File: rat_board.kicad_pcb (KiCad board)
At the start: 2 copper layers, 43.2 x 51.4 mm, 55 parts, among them M1 LEFT_MOTOR, M2 RIGHT_MOTOR, SW2 SWITCH_INV, U3 STM32F103C8T6

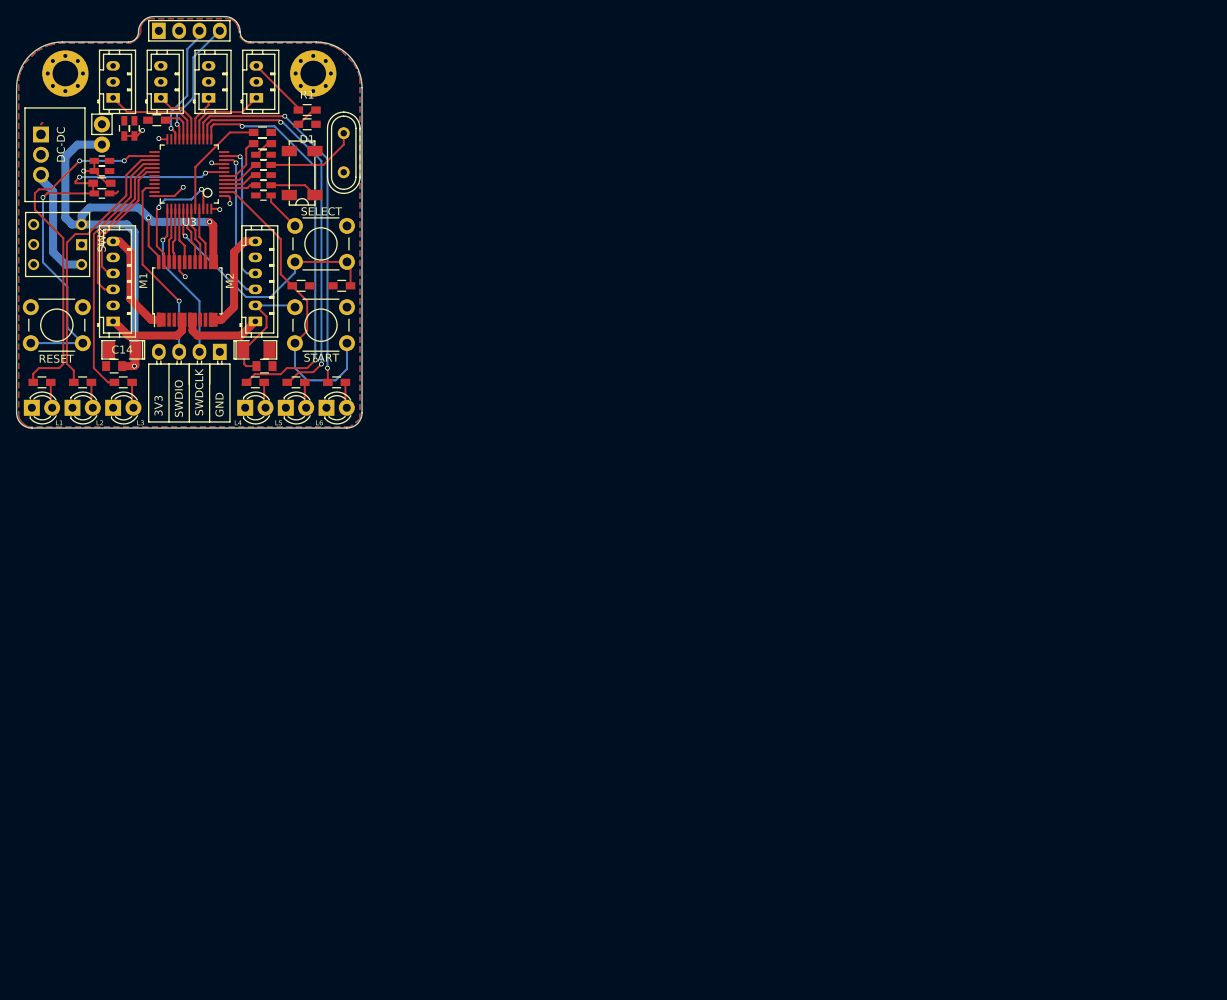
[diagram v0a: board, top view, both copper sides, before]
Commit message: releseable board
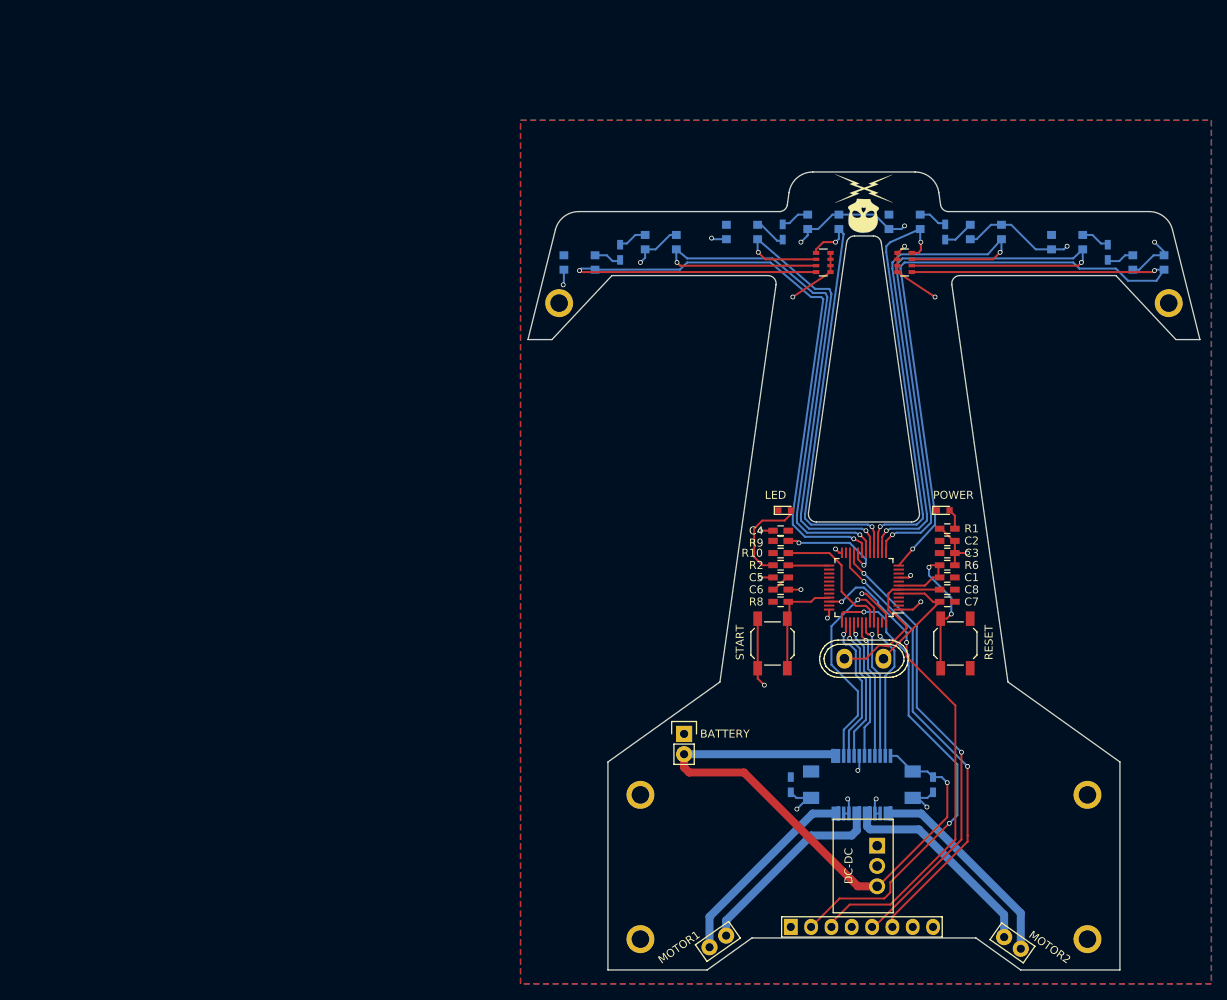
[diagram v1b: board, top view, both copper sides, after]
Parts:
- removed the ? at (75.9, 42.9)
- removed the ? at (45.7, 46.7)
- removed the ? at (38.2, 71.6)
- removed the ? at (43.3, 71.6)
- removed the ? at (48.4, 71.6)
- removed the ? at (64.9, 71.6)
- removed the ? at (75.7, 59.6)
- removed the ? at (70.6, 59.6)
- removed the ? at (65.8, 40.4)
- removed the ? at (70.0, 71.6)
- removed the ? at (75.1, 71.6)
- removed the ? at (52.8, 27.7)
- removed the ? at (65.9, 43.2)
- removed the ? at (65.9, 47.0)
- removed the ? at (65.9, 45.7)
- removed the ? at (65.0, 67.6)
- removed the ? at (45.7, 45.2)
- removed the ? at (45.7, 43.9)
- removed the ? at (65.9, 48.3)
- removed the ? at (49.8, 39.9)
- removed the ? at (48.5, 39.9)
- removed the ? at (65.9, 44.5)
- removed the ? at (45.7, 48.0)
- removed the ? at (65.8, 41.8)
- removed the ? at (52.6, 38.9)
- removed the ? at (47.2, 69.6)
- removed the ? at (66.0, 69.6)
- removed the ? at (60.5, 67.8)
- removed the ? at (41.1, 33.0)
- removed the ? at (56.4, 60.2)
- removed the ? at (70.7, 45.5)
- removed the ? at (38.1, 43.2)
- removed the ? at (72.1, 33.0)
- removed D1: LED_Power, Resistors_SMD:R_0603_HandSoldering
- removed the DC-DC at (45.7, 41.9)
- removed the G*** at (56.1, 45.0)
- removed L1: LED_0, LEDs:LED-3MM
- removed L2: LED_1, LEDs:LED-3MM
- removed L3: LED_2, LEDs:LED-3MM
- removed L4: LED_3, LEDs:LED-3MM
- removed L5: LED_4, LEDs:LED-3MM
- removed L6: LED_5, LEDs:LED-3MM
- removed M1: LEFT_MOTOR, Connectors_JST:JST_PH_B6B-PH-K_06x2.00mm_Straight
- removed M2: RIGHT_MOTOR, Connectors_JST:JST_PH_B6B-PH-K_06x2.00mm_Straight
- removed the RESET at (36.8, 62.2)
- removed S1: FRONT_LEFT_IR, Connectors_JST:JST_PH_B3B-PH-K_03x2.00mm_Straight
- removed S2: SIDE_LEFT_IR, Connectors_JST:JST_PH_B3B-PH-K_03x2.00mm_Straight
- removed S3: SIDE_RIGHT_IR, Connectors_JST:JST_PH_B3B-PH-K_03x2.00mm_Straight
- removed S4: FRONT_RIGHT_IR, Connectors_JST:JST_PH_B3B-PH-K_03x2.00mm_Straight
- removed SELECT: SELECT_BUTTON, Buttons_Switches_ThroughHole:SW_PUSH_6mm
- removed the START at (69.8, 62.2)
- removed SW2: SWITCH_INV, Buttons_Switches_ThroughHole:SW_PUSH_x2
- removed U3: STM32F103C8T6, Housings_QFP:LQFP-48_7x7mm_Pitch0.5mm
- added ?: TB6612FNG, custom-lib:driver_tuneado, B.Cu at (140.7, 121.9)
- added ?: 47k, Resistors_SMD:R_Array_Convex_4x0603, F.Cu at (146.1, 56.6)
- added ?: MountingHole_2.2mm_M2_ISO7380_Pad, Mounting_Holes:MountingHole_2.2mm_M2_ISO7380_Pad, F.Cu at (102.9, 61.7)
- added ?: MountingHole_2.2mm_M2_ISO7380_Pad, Mounting_Holes:MountingHole_2.2mm_M2_ISO7380_Pad, F.Cu at (179.1, 61.7)
- added ?: CONN_01X08, Socket_Strips:Socket_Strip_Straight_1x08, F.Cu at (131.8, 139.7)
- added ?: MountingHole_2.2mm_M2_ISO7380_Pad, Mounting_Holes:MountingHole_2.2mm_M2_ISO7380_Pad, F.Cu at (113.0, 141.2)
- added ?: MountingHole_2.2mm_M2_ISO7380_Pad, Mounting_Holes:MountingHole_2.2mm_M2_ISO7380_Pad, F.Cu at (168.9, 141.2)
- added ?: MountingHole_2.2mm_M2_ISO7380_Pad, Mounting_Holes:MountingHole_2.2mm_M2_ISO7380_Pad, F.Cu at (168.9, 123.2)
- added ?: MountingHole_2.2mm_M2_ISO7380_Pad, Mounting_Holes:MountingHole_2.2mm_M2_ISO7380_Pad, F.Cu at (113.0, 123.2)
- added ?: STM32F103C8T6, Housings_QFP:LQFP-48_7x7mm_Pitch0.5mm, F.Cu at (141.0, 97.3)
- added ?: 8MHz, Crystals:Crystal_HC50-U_Vertical, F.Cu at (141.0, 106.2)
- added ?: 47k, Resistors_SMD:R_Array_Convex_4x0603, F.Cu at (135.9, 56.6)
- added BATTERY: CONN_01X02, Socket_Strips:Socket_Strip_Straight_1x02, F.Cu at (118.5, 115.6)
- added C1: 1uF, Capacitors_SMD:C_0603_HandSoldering, F.Cu at (151.4, 96.0)
- added C11: 0.1uF, Capacitors_SMD:C_0603_HandSoldering, B.Cu at (131.8, 121.9)
- added C12: 10uF, SMD_Packages:SMD-1206_Pol, B.Cu at (134.4, 121.9)
- added C13: 0.1uF, Capacitors_SMD:C_0603_HandSoldering, B.Cu at (149.6, 121.9)
- added C2: 100nF, Capacitors_SMD:C_0603_HandSoldering, F.Cu at (151.4, 91.4)
- added C3: 100nF, Capacitors_SMD:C_0603_HandSoldering, F.Cu at (151.4, 93.0)
- added C4: 4.7uF, Capacitors_SMD:C_0603_HandSoldering, F.Cu at (130.6, 90.2)
- added C5: 10nF, Capacitors_SMD:C_0603_HandSoldering, F.Cu at (130.6, 96.0)
- added C6: 1uF, Capacitors_SMD:C_0603_HandSoldering, F.Cu at (130.6, 97.5)
- added C7: 20p, Capacitors_SMD:C_0603_HandSoldering, F.Cu at (151.4, 99.1)
- added C8: 20p, Capacitors_SMD:C_0603_HandSoldering, F.Cu at (151.4, 97.5)
- added DC-DC: TR05S3V3, custom-lib:TR05S3V3, F.Cu at (142.6, 132.1)
- added G***: LOGO, LOGO, B.Cu at (124.2, 134.6)
- added G***: LOGO, LOGO, B.Cu at (141.0, 96.5)
- added G***: LOGO, LOGO, F.Cu at (141.0, 49.3)
- added IR1: QRE1113, custom-lib:QRE1113GR, B.Cu at (105.4, 56.6)
- added IR2: QRE1113, custom-lib:QRE1113GR, B.Cu at (115.6, 54.1)
- added IR3: QRE1113, custom-lib:QRE1113GR, B.Cu at (125.7, 52.8)
- added IR4: QRE1113, custom-lib:QRE1113GR, B.Cu at (135.9, 51.6)
- added IR5: QRE1113, custom-lib:QRE1113GR, B.Cu at (146.1, 51.6)
- added IR6: QRE1113, custom-lib:QRE1113GR, B.Cu at (156.2, 52.8)
- added IR7: QRE1113, custom-lib:QRE1113GR, B.Cu at (166.4, 54.1)
- added IR8: QRE1113, custom-lib:QRE1113GR, B.Cu at (176.5, 56.6)
- added LED: LED_0, LEDs:LED_0603, F.Cu at (131.1, 87.6)
- added MOTOR1: CONN_01X02, Socket_Strips:Socket_Strip_Straight_1x02, F.Cu at (121.7, 142.2)
- added MOTOR2: CONN_01X02, Socket_Strips:Socket_Strip_Straight_1x02, F.Cu at (158.5, 141.0)
- added POWER: LED_Power, LEDs:LED_0603, F.Cu at (150.9, 87.6)
- added R10: 100k, Capacitors_SMD:C_0603_HandSoldering, F.Cu at (130.6, 93.0)
- added R13: 47, Capacitors_SMD:C_0603_HandSoldering, B.Cu at (130.8, 52.8)
- added R14: 47, Capacitors_SMD:C_0603_HandSoldering, B.Cu at (151.1, 52.8)
- added R15: 47, Capacitors_SMD:C_0603_HandSoldering, B.Cu at (171.4, 55.4)
- added R2: 100, Capacitors_SMD:C_0603_HandSoldering, F.Cu at (130.6, 94.5)
- added R6: 10k, Capacitors_SMD:C_0603_HandSoldering, F.Cu at (151.4, 94.5)
- added R7: 47, Capacitors_SMD:C_0603_HandSoldering, B.Cu at (110.5, 55.4)
- added R8: 10k, Capacitors_SMD:C_0603_HandSoldering, F.Cu at (130.6, 99.1)
- added R9: 100k, Capacitors_SMD:C_0603_HandSoldering, F.Cu at (130.6, 91.4)
- added RESET: SW_PUSH_SMALL_H, Buttons_Switches_SMD:SW_SPST_SKQG, F.Cu at (152.4, 104.3)
- added START: START_BUTTON, Buttons_Switches_SMD:SW_SPST_SKQG, F.Cu at (129.5, 104.3)
- C14: moved to B.Cu
- R1: footprint Resistors_SMD:R_0603_HandSoldering -> Capacitors_SMD:C_0603_HandSoldering
- moved C14 112.8 mm to (147.1, 121.9), turned to 270 degrees
- moved R1 95.6 mm to (151.4, 89.9)
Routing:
- net /IR7: track 0.00 -> 106.0 mm, vias 0 -> 2
- net /IR0: track 0.00 -> 101.5 mm, vias 0 -> 2
- net /IR6: track 0.00 -> 87.7 mm, vias 0 -> 2
- net /IR5: track 0.00 -> 69.0 mm, vias 0 -> 2
- net /IR1: track 12.8 -> 79.9 mm, vias 0 -> 2
- net GND: track 1.50 -> 67.2 mm, vias 0 -> 12
- net /IR2: track 7.50 -> 61.9 mm, vias 0 -> 2
- net /LED3: track 50.8 -> 0.00 mm, vias 2 -> 0
- net /LED4: track 49.0 -> 0.00 mm, vias 2 -> 0
- net /IR3: track 5.86 -> 54.2 mm, vias 0 -> 2
- net /LED5: track 48.1 -> 0.00 mm, vias 2 -> 0
- net /RX3: track 15.3 -> 56.9 mm, vias 1 -> 2
- net /IR4: track 10.7 -> 52.2 mm, vias 0 -> 2
- net /TX3: track 16.6 -> 58.0 mm, vias 1 -> 2
- net /SWDCLK: track 20.0 -> 60.0 mm, vias 1 -> 2
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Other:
- board size 43.2 x 51.4 mm -> 84 x 99.8 mm
- net class lipo: trace_width 1 -> 0.25
- net class motors: trace_width 1 -> 0.25
